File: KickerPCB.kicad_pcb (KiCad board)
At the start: 2 copper layers, 68 x 52.8 mm, 19 parts, among them J1 Conn_01x03_Pin, U1 30k, U10 N channel, U11 D, U12 10K, U13 Conn_01x02, U14 2200, U2 115k, U3 BSP89, U4 Optocoupler, U5 210, U6 2200, U7 10k, U8 210, U9 Oprocoupler

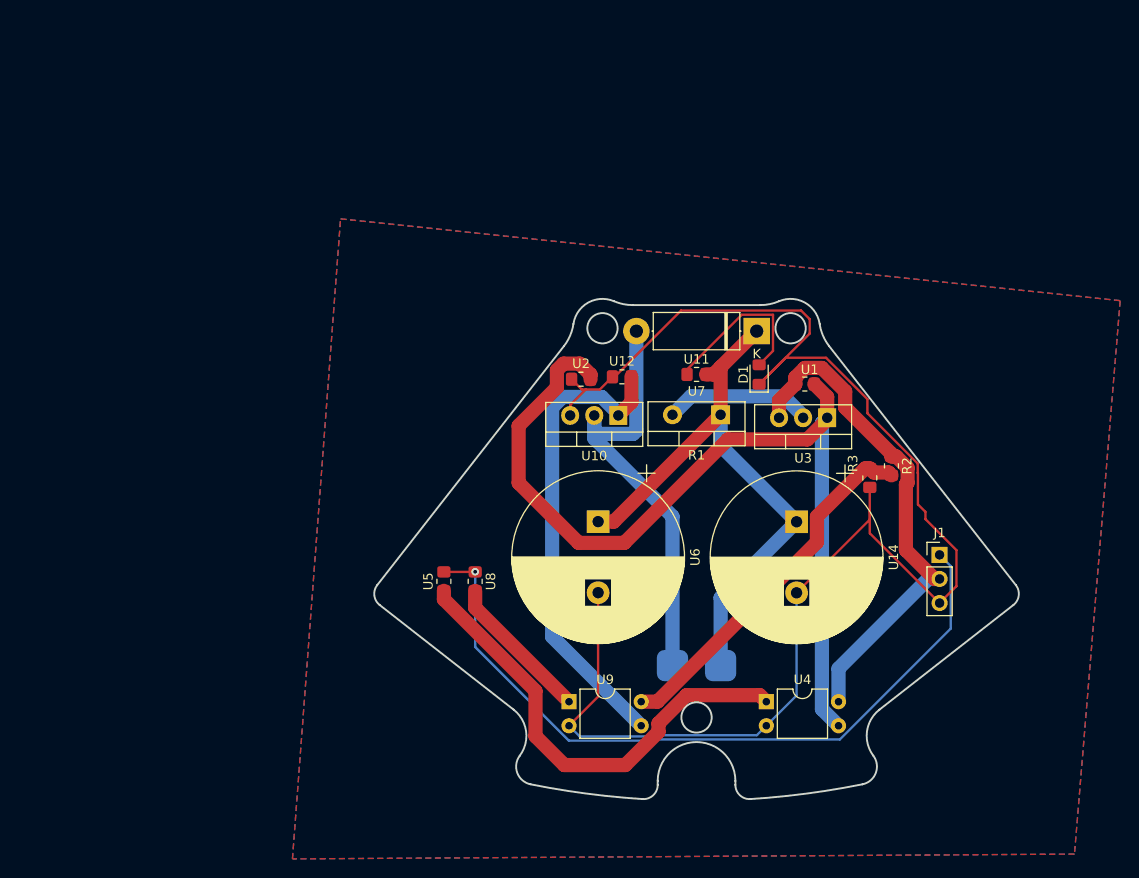
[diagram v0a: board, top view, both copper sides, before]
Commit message: Moved parts for edges
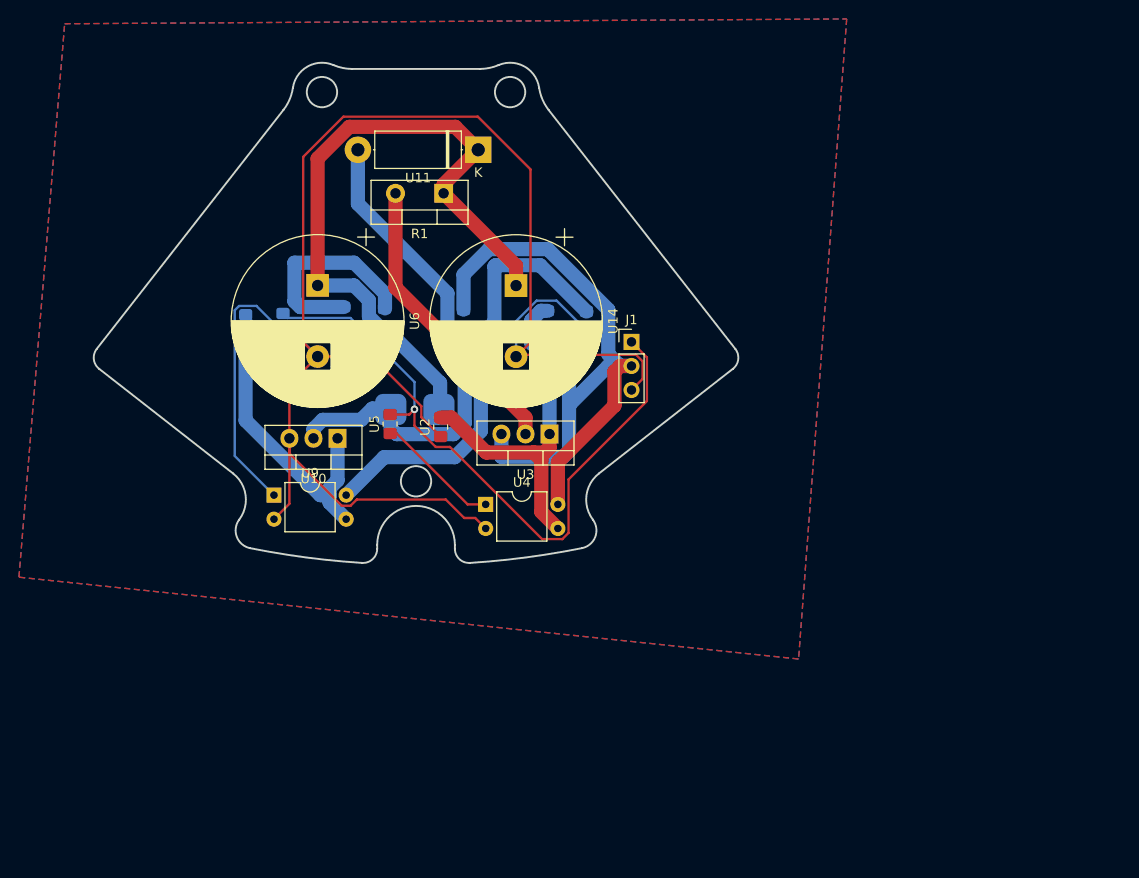
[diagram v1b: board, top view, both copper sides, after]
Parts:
- D1, R2, R3, U1, U12, U7, U8: moved to B.Cu
- moved R2 47.8 mm to (101.9, 68.5)
- moved D1 44.3 mm to (89.2, 68.2)
- moved U13 40.2 mm to (96.7, 78.0)
- moved U12 40.1 mm to (78.9, 69.0), turned to -90 degrees
- moved J1 39.5 mm to (119.6, 70.9)
- moved U14 38.7 mm to (107.4, 65.0)
- moved U6 38.7 mm to (86.5, 64.9)
- moved U9 38.0 mm to (81.9, 87.1)
- moved R1 37.4 mm to (99.8, 55.2)
- moved U4 36.2 mm to (104.2, 88.1)
- moved U11 35.1 mm to (103.4, 50.6)
- moved R3 34.2 mm to (114.8, 68.7)
- moved U8 34.0 mm to (82.8, 68.9)
- moved U7 33.5 mm to (93.5, 68.4), turned to -90 degrees
- moved U10 29.7 mm to (88.6, 81.1)
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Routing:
- net Net-(U3-G): track 96.7 -> 38.7 mm
- net Net-(U4-A): track 48.9 -> 13.2 mm
- net 48V: track 54.4 -> 80.8 mm
- net GND: track 161.9 -> 182.8 mm
- net Net-(U10-G): track 50.5 -> 30.9 mm
- net Net-(U3-D): track 15.7 -> 31.1 mm
- net Net-(U9-A): track 15.8 -> 27.7 mm
- net 12V: track 38.5 -> 49.8 mm
- net Net-(U11-K): track 63.0 -> 72.8 mm
- net Kicker: track 78.7 -> 70.1 mm
- net Net-(U10-S): track 46.6 -> 54.2 mm
- net Net-(D1-A): track 17.9 -> 22.0 mm
